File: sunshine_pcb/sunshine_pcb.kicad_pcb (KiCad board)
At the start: 2 copper layers, 82.5 x 61.9 mm, 17 parts, among them J1 XT30PW, J2 XT30PW, J3 MR30, J4 MR30, J5 USB_C_Receptacle_USB2.0_16P, SW1 Fingertech, U1 RP2350_60QFN, U2 W25Q128JVP, U3 LIS3MDL, U4 ADXL375, U5 HT7533, U6 FS2A, U7 DualAM32

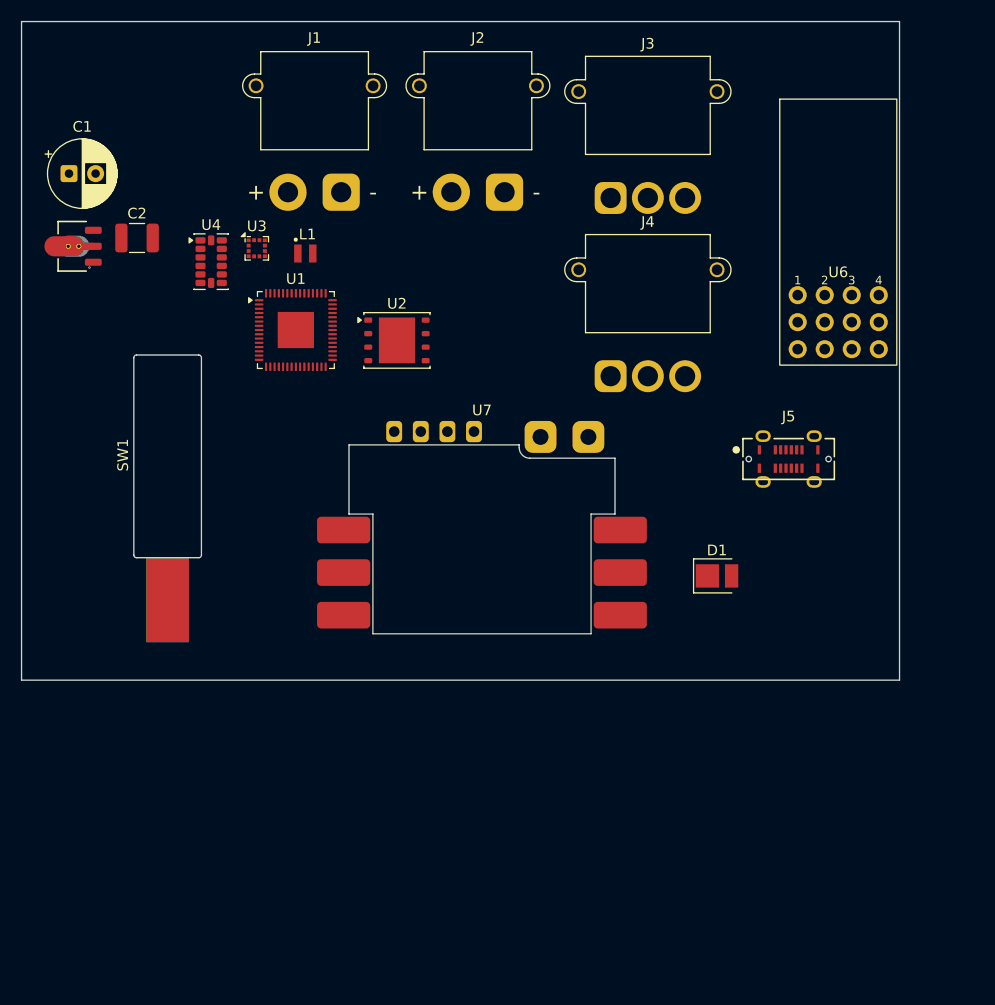
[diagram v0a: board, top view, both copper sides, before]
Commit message: Do layout
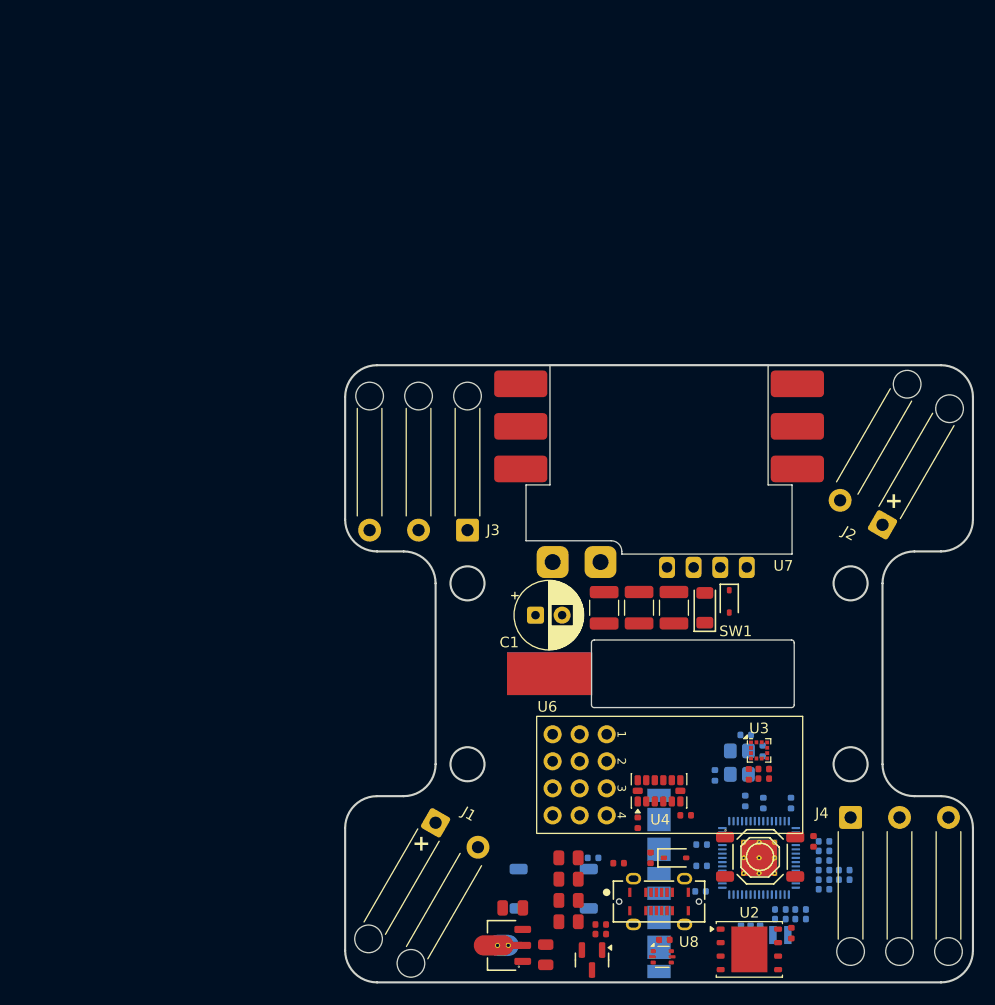
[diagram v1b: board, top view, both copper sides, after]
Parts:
- added C10: 100nF, PCM_JLCPCB:C_0402, B.Cu at (104.0, 118.0)
- added C11: 100nF, PCM_JLCPCB:C_0402, B.Cu at (115.5, 116.7)
- added C12: 4.7uF, PCM_JLCPCB:C_0402, B.Cu at (109.8, 112.2)
- added C13: 100nF, PCM_JLCPCB:C_0402, B.Cu at (115.5, 120.2)
- added C14: 100nF, PCM_JLCPCB:C_0402, B.Cu at (115.5, 115.8)
- added C15: 100nF, PCM_JLCPCB:C_0402, B.Cu at (112.4, 112.2)
- added C16: 100nF, PCM_JLCPCB:C_0402, B.Cu at (108.1, 112.0)
- added C17: 100nF, PCM_JLCPCB:C_0402, B.Cu at (104.0, 116.0)
- added C18: 100nF, PCM_JLCPCB:C_0402, B.Cu at (103.9, 120.5)
- added C19: 100nF, PCM_JLCPCB:C_0402, B.Cu at (107.7, 124.2)
- added C22: 100nF, PCM_JLCPCB:C_0402, F.Cu at (112.4, 124.4)
- added C23: 15pF, PCM_JLCPCB:C_0402, B.Cu at (105.2, 109.5)
- added C24: 15pF, PCM_JLCPCB:C_0402, B.Cu at (108.2, 105.8)
- added C25: 100nF, PCM_JLCPCB:C_0402, F.Cu at (102.5, 113.3)
- added C26: 100nF, PCM_JLCPCB:C_0402, F.Cu at (98.0, 114.0)
- added C27: 100nF, PCM_JLCPCB:C_0402, F.Cu at (108.4, 109.5)
- added C28: 100nF, PCM_JLCPCB:C_0402, F.Cu at (109.8, 109.0)
- added C29: 4.7uF, PCM_JLCPCB:C_0402, F.Cu at (109.8, 109.8)
- added C3: 10u, Capacitor_SMD:C_1210_3225Metric, F.Cu at (94.8, 93.8)
- added C30: 100nF, PCM_JLCPCB:C_0402, B.Cu at (115.5, 117.5)
- added C4: 10u, Capacitor_SMD:C_1210_3225Metric, F.Cu at (101.4, 93.8)
- added C5: 10uF, PCM_JLCPCB:C_0805, F.Cu at (89.3, 126.4)
- added C6: 10uF, PCM_JLCPCB:C_0805, F.Cu at (86.2, 122.0)
- added C7: 4.7uF, PCM_JLCPCB:C_0402, B.Cu at (113.3, 123.0)
- added C8: 4.7uF, PCM_JLCPCB:C_0402, B.Cu at (111.4, 122.2)
- added C9: 4.7uF, PCM_JLCPCB:C_0402, B.Cu at (111.4, 123.0)
- added D2: 1N5819WS, PCM_JLCPCB:D_SOD-323, F.Cu at (106.6, 93.2)
- added D3: 1N5819WS, PCM_JLCPCB:D_SOD-323, F.Cu at (101.5, 117.3)
- added D4: LED, LED_SMD:LED_PLCC_2835, B.Cu at (100.0, 122.0)
- added D5: LED, LED_SMD:LED_PLCC_2835, B.Cu at (100.0, 112.8)
- added D6: LED, LED_SMD:LED_PLCC_2835, B.Cu at (100.0, 117.4)
- added D7: SMF12A, PCM_JLCPCB:D_SOD-123FL, F.Cu at (104.3, 93.8)
- added Q1: AO3401A, PCM_JLCPCB:Q_SOT-23, F.Cu at (93.7, 126.9)
- added R1: 5.1kΩ, PCM_JLCPCB:R_0402, F.Cu at (99.2, 117.3)
- added R10: 33Ω, PCM_JLCPCB:R_0805, F.Cu at (91.5, 123.3)
- added R11: 1kΩ, PCM_JLCPCB:R_0402, F.Cu at (94.5, 123.6)
- added R12: 33Ω, PCM_JLCPCB:R_0805, F.Cu at (91.5, 121.3)
- added R13: 33Ω, PCM_JLCPCB:R_0805, F.Cu at (91.5, 117.3)
- added R14: 33Ω, PCM_JLCPCB:R_0805, F.Cu at (91.5, 119.3)
- added R15: 5.1kΩ, PCM_JLCPCB:R_0402, B.Cu at (115.5, 119.3)
- added R16: 5.1kΩ, PCM_JLCPCB:R_0402, B.Cu at (117.4, 119.3)
- added R17: 5.1kΩ, PCM_JLCPCB:R_0402, B.Cu at (115.5, 118.5)
- added R18: 1kΩ, PCM_JLCPCB:R_0402, B.Cu at (117.4, 118.5)
- added R19: 5.1kΩ, PCM_JLCPCB:R_0402, F.Cu at (94.5, 124.5)
- added R2: 5.1kΩ, PCM_JLCPCB:R_0402, F.Cu at (100.5, 125.0)
- added R3: 5.1kΩ, PCM_JLCPCB:R_0402, F.Cu at (96.2, 117.8)
- added R4: 33Ω, PCM_JLCPCB:R_0402, B.Cu at (113.3, 122.2)
- added R5: 33Ω, PCM_JLCPCB:R_0402, B.Cu at (108.6, 124.2)
- added R6: 33Ω, PCM_JLCPCB:R_0402, B.Cu at (109.5, 124.2)
- added R7: 1kΩ, PCM_JLCPCB:R_0402, B.Cu at (93.8, 117.3)
- added R8: 1kΩ, PCM_JLCPCB:R_0402, B.Cu at (109.8, 107.2)
- added R9: 1kΩ, PCM_JLCPCB:R_0402, F.Cu at (114.5, 115.8)
- added S1: TS-1187A-C-B-B, PCM_JLCPCB:SW-SMD_4P-L5.1-W5.1-P3.70-LS6.5-TL-2, B.Cu at (90.1, 120.2)
- added S2: TS-1187A-C-B-B, PCM_JLCPCB:SW-SMD_4P-L5.1-W5.1-P3.70-LS6.5-TL-2, F.Cu at (109.5, 117.2)
- added U8: USBLC6-2P6, Package_TO_SOT_SMD:SOT-666, F.Cu at (100.3, 126.6)
- added Y1: ABM8-272-T3, Crystal:Crystal_SMD_3225-4Pin_3.2x2.5mm, B.Cu at (107.5, 108.3)
- D1: moved to B.Cu
- J1, J2: value XT30PW -> Soldered; footprint Connector_AMASS:AMASS_XT30PW-M_1x02_P2.50mm_Horizontal -> Connector_Wire:SolderWire-0.5sqmm_1x02_P4.6mm_D0.9mm_OD2.1mm_Relief
- J3, J4: value MR30 -> Soldered; footprint Connector_AMASS:AMASS_MR30PW-M_1x03_P3.50mm_Horizontal -> Connector_Wire:SolderWire-0.5sqmm_1x03_P4.6mm_D0.9mm_OD2.1mm_Relief
- J5: value USB_C_Receptacle_USB2.0_16P -> VerticalUSB
- L1: value L -> 3.3u; moved to B.Cu
- U1: footprint Package_DFN_QFN:QFN-60-1EP_7x7mm_P0.4mm_EP3.4x3.4mm -> Package_DFN_QFN:QFN-60-1EP_7x7mm_P0.4mm_EP3.4x3.4mm_ThermalVias; moved to B.Cu
- moved L1 78.1 mm to (111.4, 124.5)
- moved U5 77.1 mm to (85.8, 125.5)
- moved U3 66.7 mm to (109.4, 107.2)
- moved U2 66.1 mm to (108.5, 125.9)
- moved U1 66.0 mm to (109.4, 117.3)
- moved U4 65.2 mm to (100.0, 111.0), turned to 90 degrees
- moved J1 62.7 mm to (79.0, 114.0), turned to -30 degrees
- moved C1 60.4 mm to (88.4, 94.5)
- moved C2 58.6 mm to (98.1, 93.8), turned to 90 degrees
- moved J2 50.8 mm to (121.0, 86.0), turned to 150 degrees
- moved SW1 49.3 mm to (100.0, 100.0), turned to 0 degrees
- moved J4 47.2 mm to (118.0, 113.5)
- moved U6 46.4 mm to (90.0, 108.2), turned to -90 degrees
- moved J5 43.3 mm to (100.0, 121.4)
- moved D1 36.2 mm to (100.0, 126.6), turned to -90 degrees
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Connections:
- net Net-(J5-VBUS-PadA4) renamed VBUS
- C1 pad 1: unconnected-(C1-Pad1) -> VDC
- C1 pad 2: unconnected-(C1-Pad2) -> GND
- C2 pad 1: unconnected-(C2-Pad1) -> VDC
- C2 pad 2: unconnected-(C2-Pad2) -> GND
- D1 pad 1: unconnected-(D1-K-Pad1) -> GND
- D1 pad 2: unconnected-(D1-A-Pad2) -> Net-(D1-A)
- J1 pad 1: unconnected-(J1---Pad1) -> /BATT1_+
- J1 pad 2: unconnected-(J1-+-Pad2) -> /BATT2_+
- J2 pad 1: unconnected-(J2---Pad1) -> /BATT2_+
- J2 pad 2: unconnected-(J2-+-Pad2) -> GND
- J3 pad 1: unconnected-(J3-Pin_1-Pad1) -> Net-(J3-Pin_1)
- J3 pad 2: unconnected-(J3-Pin_2-Pad2) -> Net-(J3-Pin_2)
- J3 pad 3: unconnected-(J3-Pin_3-Pad3) -> Net-(J3-Pin_3)
- J4 pad 1: unconnected-(J4-Pin_1-Pad1) -> Net-(J4-Pin_1)
- J4 pad 2: unconnected-(J4-Pin_2-Pad2) -> Net-(J4-Pin_2)
- J4 pad 3: unconnected-(J4-Pin_3-Pad3) -> Net-(J4-Pin_3)
- J5 pad A1: Net-(J5-GND-PadA1) -> GND
- J5 pad A12: Net-(J5-GND-PadA1) -> GND
- J5 pad A5: unconnected-(J5-CC1-PadA5) -> Net-(J5-CC1)
- J5 pad A6: unconnected-(J5-D+-PadA6) -> /USB_C_D+
- J5 pad A7: unconnected-(J5-D--PadA7) -> /USB_C_D-
- J5 pad B1: Net-(J5-GND-PadA1) -> GND
- J5 pad B12: Net-(J5-GND-PadA1) -> GND
- J5 pad B5: unconnected-(J5-CC2-PadB5) -> Net-(J5-CC2)
- J5 pad B6: unconnected-(J5-D+-PadB6) -> /USB_C_D+
- J5 pad B7: unconnected-(J5-D--PadB7) -> /USB_C_D-
- J5 pad S1: unconnected-(J5-SHIELD-PadS1) -> Net-(J5-SHIELD)
- L1 pad 1: unconnected-(L1-Pad1) -> +1V1
- L1 pad 2: unconnected-(L1-Pad2) -> /VREG_LX
- SW1 pad 1: unconnected-(SW1-A-Pad1) -> /BATT1_+
- SW1 pad 2: unconnected-(SW1-B-Pad2) -> VDC
- U1 pad 1: unconnected-(U1-IOVDD-Pad1) -> +3V3
- U1 pad 10: unconnected-(U1-GPIO7-Pad10) -> /R4
- U1 pad 11: unconnected-(U1-IOVDD-Pad11) -> +3V3
- U1 pad 12: unconnected-(U1-GPIO8-Pad12) -> /S2
- U1 pad 13: unconnected-(U1-GPIO9-Pad13) -> /LED
- U1 pad 14: unconnected-(U1-GPIO10-Pad14) -> /IMU_SCK
- U1 pad 15: unconnected-(U1-GPIO11-Pad15) -> /IMU_MOSI
- U1 pad 16: unconnected-(U1-GPIO12-Pad16) -> /IMU_MISO
- U1 pad 17: unconnected-(U1-GPIO13-Pad17) -> /IMU_CS
- U1 pad 18: unconnected-(U1-GPIO14-Pad18) -> /IMU_INT1
- U1 pad 19: unconnected-(U1-GPIO15-Pad19) -> /IMU_INT2
- U1 pad 20: unconnected-(U1-IOVDD-Pad20) -> +3V3
- U1 pad 21: unconnected-(U1-XIN-Pad21) -> Net-(U1-XIN)
- U1 pad 22: unconnected-(U1-XOUT-Pad22) -> Net-(U1-XOUT)
- U1 pad 23: unconnected-(U1-DVDD-Pad23) -> +1V1
- U1 pad 26: unconnected-(U1-RUN-Pad26) -> /RESET
- U1 pad 27: unconnected-(U1-GPIO16-Pad27) -> /MAG_MISO
- U1 pad 28: unconnected-(U1-GPIO17-Pad28) -> /MAG_CS
- U1 pad 29: unconnected-(U1-GPIO18-Pad29) -> /MAG_SCK
- U1 pad 3: unconnected-(U1-GPIO1-Pad3) -> /R1
- U1 pad 30: unconnected-(U1-IOVDD-Pad30) -> +3V3
- U1 pad 31: unconnected-(U1-GPIO19-Pad31) -> /MAG_MOSI
- U1 pad 32: unconnected-(U1-GPIO20-Pad32) -> /MAG_DRDY
- U1 pad 33: unconnected-(U1-GPIO21-Pad33) -> /MAG_INT
- U1 pad 38: unconnected-(U1-IOVDD-Pad38) -> +3V3
- U1 pad 39: unconnected-(U1-DVDD-Pad39) -> +1V1
- U1 pad 40: unconnected-(U1-GPIO26_ADC0-Pad40) -> Net-(U1-GPIO26_ADC0)
- U1 pad 44: unconnected-(U1-ADC_AVDD-Pad44) -> +3V3
- U1 pad 45: unconnected-(U1-IOVDD-Pad45) -> +3V3
- U1 pad 46: unconnected-(U1-VREG_AVDD-Pad46) -> /VREG_AVDD
- U1 pad 47: unconnected-(U1-VREG_PGND-Pad47) -> GND
- U1 pad 48: unconnected-(U1-VREG_LX-Pad48) -> /VREG_LX
- U1 pad 49: unconnected-(U1-VREG_VIN-Pad49) -> +3V3
- U1 pad 5: unconnected-(U1-GPIO3-Pad5) -> /R2
- U1 pad 50: unconnected-(U1-VREG_FB-Pad50) -> +1V1
- U1 pad 51: unconnected-(U1-USB_DM-Pad51) -> Net-(U1-USB_DM)
- U1 pad 52: unconnected-(U1-USB_DP-Pad52) -> Net-(U1-USB_DP)
- U1 pad 53: unconnected-(U1-USB_OTP_VDD-Pad53) -> +3V3
- U1 pad 54: unconnected-(U1-QSPI_IOVDD-Pad54) -> +3V3
- U1 pad 55: unconnected-(U1-QSPI_SD3-Pad55) -> /QSPI_SD3
- U1 pad 56: unconnected-(U1-QSPI_SCLK-Pad56) -> /QSPI_SCK
- U1 pad 57: unconnected-(U1-QSPI_SD0-Pad57) -> /QSPI_SD0
- U1 pad 58: unconnected-(U1-QSPI_SD2-Pad58) -> /QSPI_SD2
- U1 pad 59: unconnected-(U1-QSPI_SD1-Pad59) -> /QSPI_SD1
- U1 pad 6: unconnected-(U1-DVDD-Pad6) -> +1V1
- U1 pad 60: unconnected-(U1-QSPI_SS-Pad60) -> /QSPI_SS
- U1 pad 61: unconnected-(U1-GND-Pad61) -> GND
- U1 pad 8: unconnected-(U1-GPIO5-Pad8) -> /R3
- U1 pad 9: unconnected-(U1-GPIO6-Pad9) -> /S1
- U2 pad 1: unconnected-(U2-~{CS}-Pad1) -> /QSPI_SS
- U2 pad 2: unconnected-(U2-DO/IO_{1}-Pad2) -> /QSPI_SD1
- U2 pad 3: unconnected-(U2-~{WP}/IO_{2}-Pad3) -> /QSPI_SD2
- U2 pad 4: unconnected-(U2-GND-Pad4) -> GND
- U2 pad 5: unconnected-(U2-DI/IO_{0}-Pad5) -> /QSPI_SD0
- U2 pad 6: unconnected-(U2-CLK-Pad6) -> /QSPI_SCK
- U2 pad 7: unconnected-(U2-~{HOLD}/~{RESET}/IO_{3}-Pad7) -> /QSPI_SD3
- U2 pad 8: unconnected-(U2-VCC-Pad8) -> +3V3
- U2 pad 9: unconnected-(U2-EP-Pad9) -> GND
- U3 pad 1: unconnected-(U3-SCL/SPC-Pad1) -> /MAG_SCK
- U3 pad 10: unconnected-(U3-~{CS}-Pad10) -> /MAG_CS
- U3 pad 11: unconnected-(U3-SDA/SDI/SDO-Pad11) -> /MAG_MOSI
- U3 pad 12: Net-(U3-GND-Pad12) -> GND
- U3 pad 2: Net-(U3-GND-Pad12) -> GND
- U3 pad 3: Net-(U3-GND-Pad12) -> GND
- U3 pad 4: unconnected-(U3-C1-Pad4) -> Net-(U3-C1)
- U3 pad 5: unconnected-(U3-Vdd-Pad5) -> +3V3
- U3 pad 6: unconnected-(U3-Vdd_IO-Pad6) -> +3V3
- U3 pad 7: unconnected-(U3-INT-Pad7) -> /MAG_INT
- U3 pad 8: unconnected-(U3-DRDY-Pad8) -> /MAG_DRDY
- U3 pad 9: unconnected-(U3-SDO/SA1-Pad9) -> /MAG_MISO
- U4 pad 1: unconnected-(U4-Vdd_I/O-Pad1) -> +3V3
- U4 pad 12: unconnected-(U4-SDO/ADDR-Pad12) -> /IMU_MISO
- U4 pad 13: unconnected-(U4-SDA/SDI/SDIO-Pad13) -> /IMU_MOSI
- U4 pad 14: unconnected-(U4-SCL/SCLK-Pad14) -> /IMU_SCK
- U4 pad 2: Net-(U4-GND-Pad2) -> GND
- U4 pad 4: Net-(U4-GND-Pad2) -> GND
- U4 pad 5: Net-(U4-GND-Pad2) -> GND
- U4 pad 6: unconnected-(U4-Vs-Pad6) -> +3V3
- U4 pad 7: unconnected-(U4-~{CS}-Pad7) -> /IMU_CS
- U4 pad 8: unconnected-(U4-INT1-Pad8) -> /IMU_INT1
- U4 pad 9: unconnected-(U4-INT2-Pad9) -> /IMU_INT2
- U5 pad 1: unconnected-(U5-GND-Pad1) -> GND
- U5 pad 2: unconnected-(U5-VIN-Pad2) -> +5V
- U5 pad 3: unconnected-(U5-VOUT-Pad3) -> +3V3
- U6 pad 1: unconnected-(U6-Pad1) -> /R1
- U6 pad 2: unconnected-(U6-Pad2) -> /R2
- U6 pad 3: unconnected-(U6-Pad3) -> /R3
- U6 pad 4: unconnected-(U6-Pad4) -> /R4
- U6 pad 5: unconnected-(U6-+5V-Pad5) -> +5V
- U6 pad 6: unconnected-(U6-GND-Pad6) -> GND
- U7 pad 1: unconnected-(U7-M1A-Pad1) -> Net-(J3-Pin_3)
- U7 pad 10: unconnected-(U7-S2-Pad10) -> /S2
- U7 pad 11: unconnected-(U7-+5V-Pad11) -> Net-(U7-+5V)
- U7 pad 12: Net-(U7-GND-Pad12) -> GND
- U7 pad 2: unconnected-(U7-M1B-Pad2) -> Net-(J3-Pin_2)
- U7 pad 3: unconnected-(U7-M1C-Pad3) -> Net-(J3-Pin_1)
- U7 pad 4: unconnected-(U7-M2A-Pad4) -> Net-(J4-Pin_1)
- U7 pad 5: unconnected-(U7-M2B-Pad5) -> Net-(J4-Pin_2)
- U7 pad 6: unconnected-(U7-M2C-Pad6) -> Net-(J4-Pin_3)
- U7 pad 7: unconnected-(U7-+VDC-Pad7) -> VDC
- U7 pad 8: Net-(U7-GND-Pad12) -> GND
- U7 pad 9: unconnected-(U7-S1-Pad9) -> /S1
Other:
- board size 82.5 x 61.9 mm -> 59 x 58 mm
- board text added: "+"
